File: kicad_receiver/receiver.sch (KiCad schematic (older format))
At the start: 51 parts, among them J1 Conn_01x05_Male, J2 M1+, J3 M1-, J4 M2+, J5 M2-, J6 CHG+5V, J7 CHG-, J8 BAT+, J9 BAT-, U1 LP2985-3.3, U10 4N26, U11 4N26, U2 STM32F030F4Px, U3 NRF24L01_Breakout, U4 LP2985-3.3, U5 L9110, U6 L9110, U7 TP4056, U8 4N26, U9 4N26

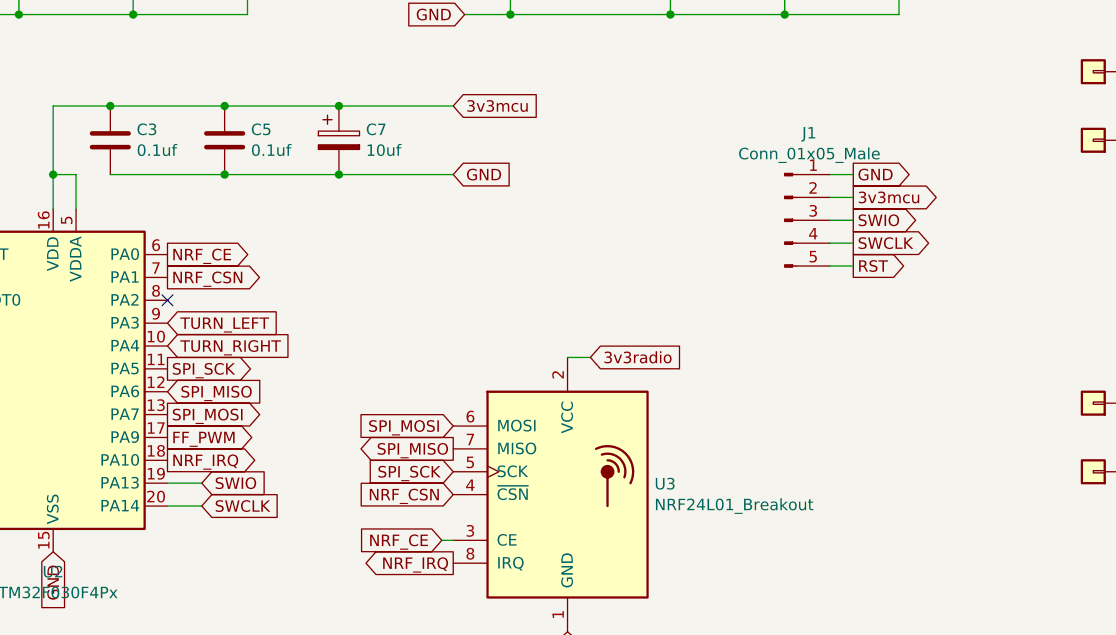
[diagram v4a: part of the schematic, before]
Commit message: done!
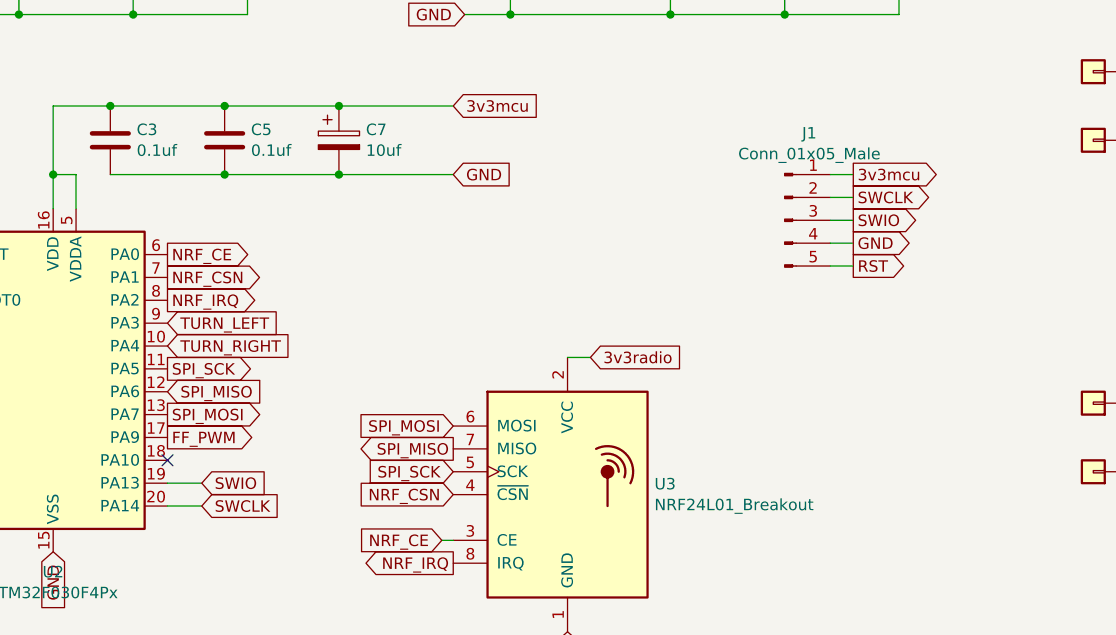
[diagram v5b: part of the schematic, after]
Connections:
- net 3v3mcu: now also J1.1 (Pin_1); no longer J1.2 (Pin_2)
- net GND: now also J1.4 (Pin_4); no longer J1.1 (Pin_1)
- net NRF_IRQ: now also U2.8 (PA2); no longer U2.18 (PA10)
- net SWCLK: now also J1.2 (Pin_2); no longer J1.4 (Pin_4)
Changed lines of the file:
@@
 Text GLabel 5500 2500 2    50   Output ~ 0
 RST
-Text GLabel 5500 2400 2    50   Output ~ 0
+Text GLabel 5500 2200 2    50   Output ~ 0
 SWCLK
 Wire Wire Line
@@
 Text GLabel 2650 3550 2    50   Input ~ 0
 SWCLK
-Text GLabel 5500 2200 2    50   Output ~ 0
+Text GLabel 5500 2100 2    50   Output ~ 0
 3v3mcu
-Text GLabel 5500 2100 2    50   Output ~ 0
+Text GLabel 5500 2400 2    50   Output ~ 0
 GND
 Wire Wire Line
@@
 Wire Wire Line
 	3700 3700 3750 3700
-NoConn ~ 2500 2650
+NoConn ~ 2500 3350
 Wire Wire Line
 	4000 1400 4700 1400
@@
 Text GLabel 3750 3800 0    50   Output ~ 0
 NRF_IRQ
-Text GLabel 2500 3350 2    50   Output ~ 0
+Text GLabel 2500 2650 2    50   Output ~ 0
 NRF_IRQ
 Text GLabel 2500 2450 2    50   Output ~ 0
